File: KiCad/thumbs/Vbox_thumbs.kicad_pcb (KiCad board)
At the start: 2 copper layers, 33.1 x 114.3 mm, 4 parts, among them J4 Conn_01x06, J5 Conn_01x06, J6 Conn_01x10, J7 Conn_01x10

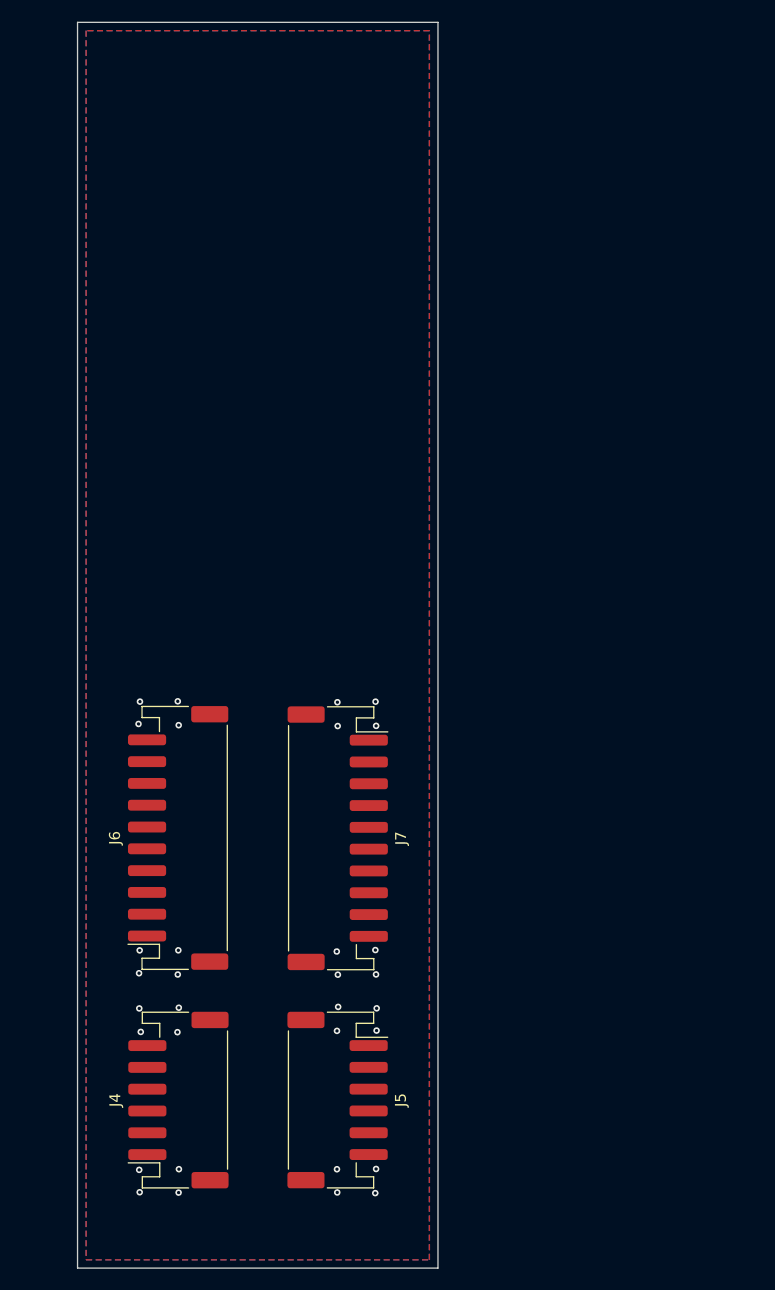
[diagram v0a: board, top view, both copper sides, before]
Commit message: thumbs and fingers
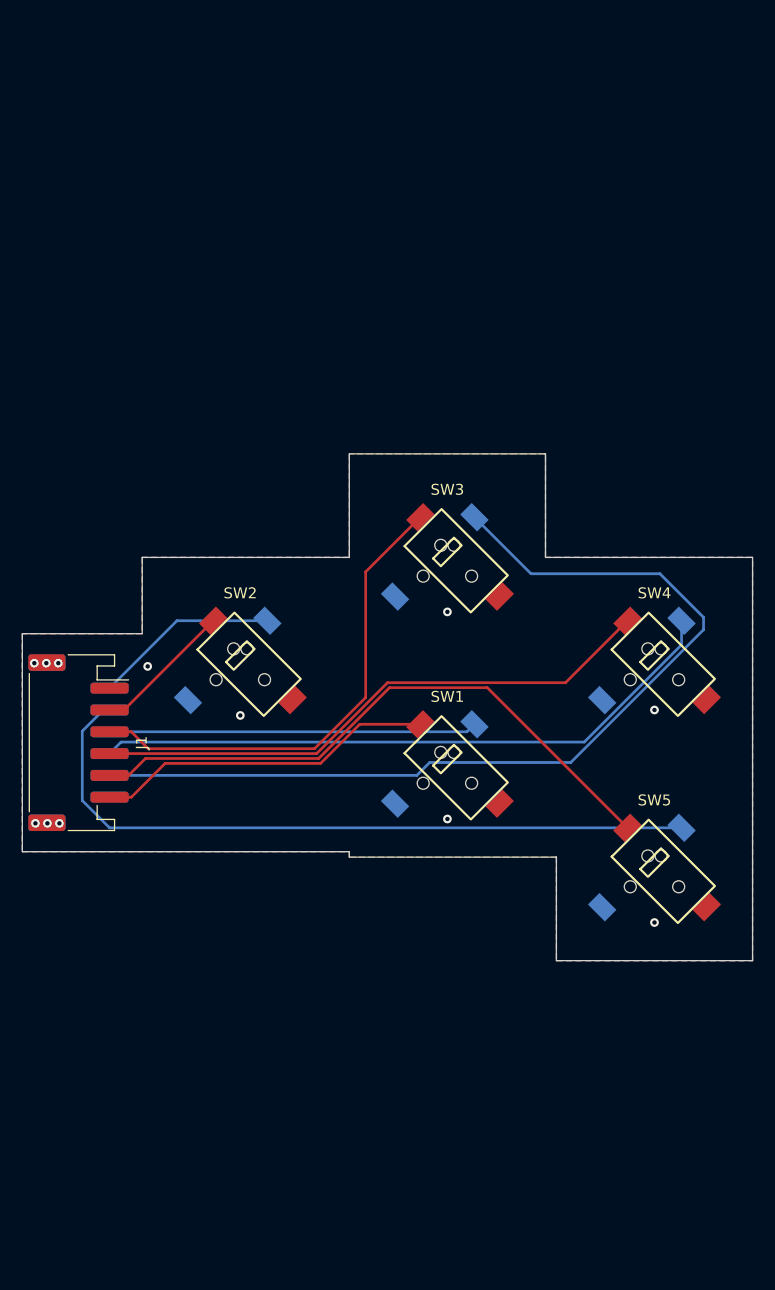
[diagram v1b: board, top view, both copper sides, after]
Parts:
- removed J4, J5: Conn_01x06, Connector_JST:JST_PH_S6B-PH-SM4-TB_1x06-1MP_P2.00mm_Horizontal
- removed J6, J7: Conn_01x10, Connector_JST:JST_PH_S10B-PH-SM4-TB_1x10-1MP_P2.00mm_Horizontal
- added J1: Conn_01x06, Connector_JST:JST_PH_S6B-PH-SM4-TB_1x06-1MP_P2.00mm_Horizontal, F.Cu at (85.2, 108.0)
- added J2: Conn_01x06, Connector_JST:JST_PH_S6B-PH-SM4-TB_1x06-1MP_P2.00mm_Horizontal, B.Cu at (85.2, 108.0)
- added SW1: SW_Push_45deg, Buttons:Vbox, F.Cu at (119.0, 109.5)
- added SW10: SW_Push_45deg, Buttons:Vbox, B.Cu at (138.0, 119.0)
- added SW2: SW_Push_45deg, Buttons:Vbox, F.Cu at (100.0, 100.0)
- added SW3: SW_Push_45deg, Buttons:Vbox, F.Cu at (119.0, 90.5)
- added SW4: SW_Push_45deg, Buttons:Vbox, F.Cu at (138.0, 100.0)
- added SW5: SW_Push_45deg, Buttons:Vbox, F.Cu at (138.0, 119.0)
- added SW6: SW_Push_45deg, Buttons:Vbox, B.Cu at (119.0, 109.5)
- added SW7: SW_Push_45deg, Buttons:Vbox, B.Cu at (100.0, 100.0)
- added SW8: SW_Push_45deg, Buttons:Vbox, B.Cu at (119.0, 90.5)
- added SW9: SW_Push_45deg, Buttons:Vbox, B.Cu at (138.0, 100.0)
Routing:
- net C_UP: track 0.00 -> 86.0 mm
- net C_DN: track 0.00 -> 65.7 mm
- net C_LT: track 0.00 -> 58.8 mm
- net M2: track 0.00 -> 56.2 mm
- net M3: track 0.00 -> 52.6 mm
- net M4: track 0.00 -> 44.7 mm
- net A: track 0.00 -> 33.8 mm
- net M1: track 0.00 -> 31.3 mm
- net C_RT: track 0.00 -> 17.0 mm
- net M5: track 0.00 -> 12.9 mm
- net GND: vias 32 -> 12
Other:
- board size 33.1 x 114.3 mm -> 67 x 46.5 mm
